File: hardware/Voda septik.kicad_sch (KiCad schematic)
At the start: 39 parts, among them J1 Screw_Terminal_01x09, J2 RS-485 elektroměr, J3 Display TM1637, J4 Display LCD I2C, U1 ESP32-DevKitC, U2 DC-DC 24V -> 5V, U4 MAX3485-modul

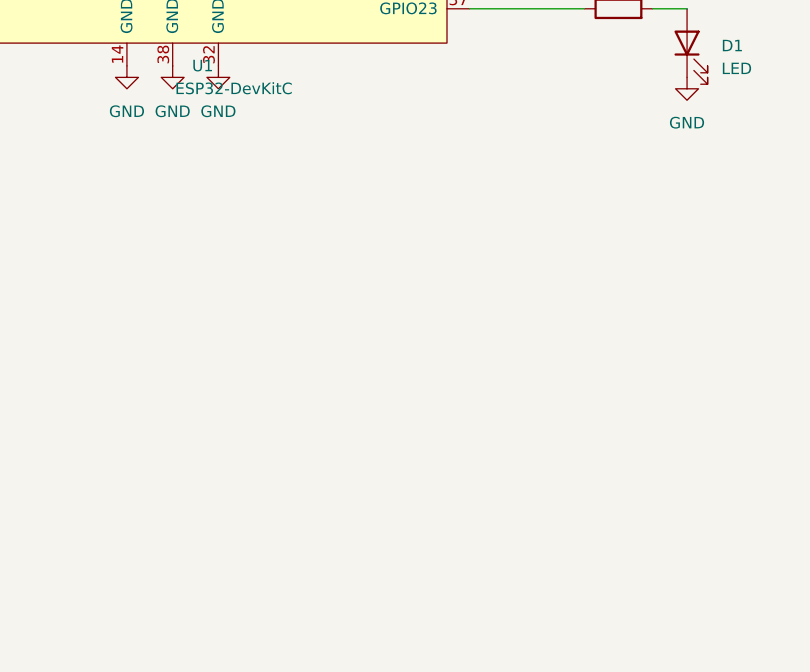
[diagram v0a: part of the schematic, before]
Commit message: Úprava schématu, asi popisky.
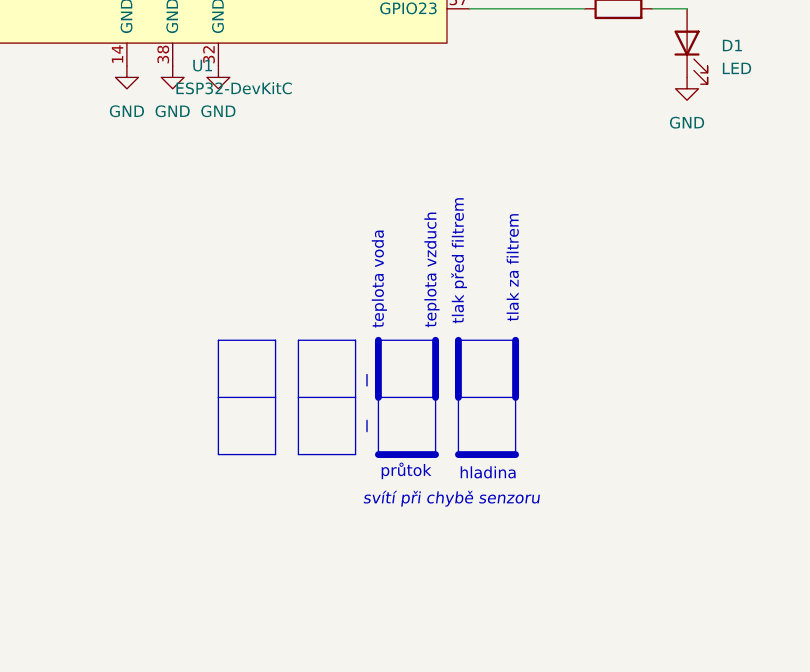
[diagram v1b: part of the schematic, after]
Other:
- note added: "hladina"
- note added: "průtok"
- note added: "svítí při chybě senzoru"
- note added: "teplota voda"
- note added: "teplota vzduch"
- note added: "tlak před filtrem"
- note added: "tlak za filtrem"
